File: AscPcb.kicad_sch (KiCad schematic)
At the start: 92 parts, among them J1 12402012E212A, J10 Conn_01x02_Pin, J11 Conn_01x02_Pin, J12 Conn_01x02_Pin, J13 Conn_01x02_Pin, J14 Conn_01x02_Pin, J15 Conn_01x02_Pin, J16 Conn_01x02_Pin, J17 Conn_01x02_Pin, J2 B2B-PH-K-S(LF)(SN), J3 Screw_Terminal_01x02, J4 Screw_Terminal_01x02, J5 Conn_01x15_Pin, J6 Conn_01x06_Pin, J7 Conn_01x02_Pin, J8 Conn_01x02_Pin, Q1 Q_NMOS_DGS, Q2 BC817, Q3 BC817, SW1 TL3305AF260QG, SW2 TL3305AF260QG, U1 BQ24040DSQR, U2 TLV75801PDRVR, U3 AP62300TWU, U4 LTC3625EDE_PBF, U5 ESP32-C3-WROOM-02-N4, U6 CP2102N-A02-GQFN24R, U7 BMI270, U8 74LVC1G07

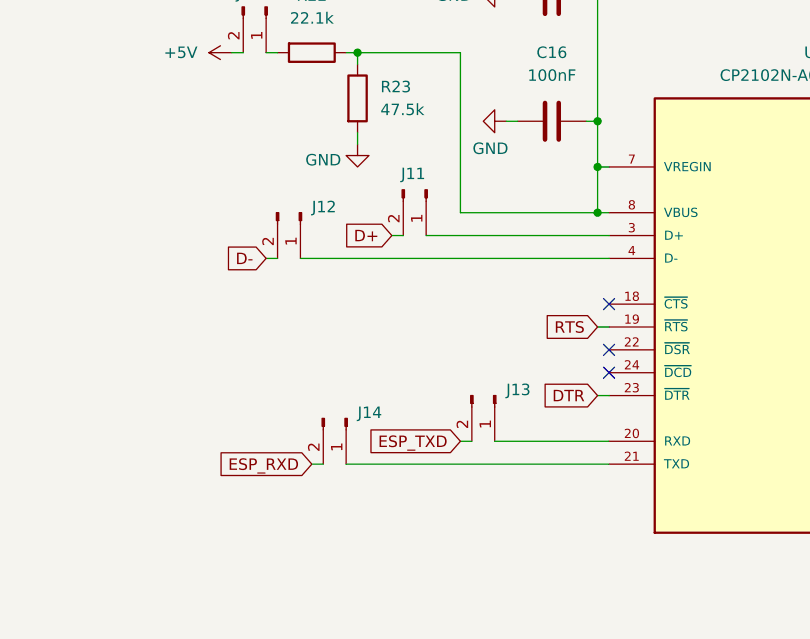
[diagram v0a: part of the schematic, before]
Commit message: first attempt at putting down traces
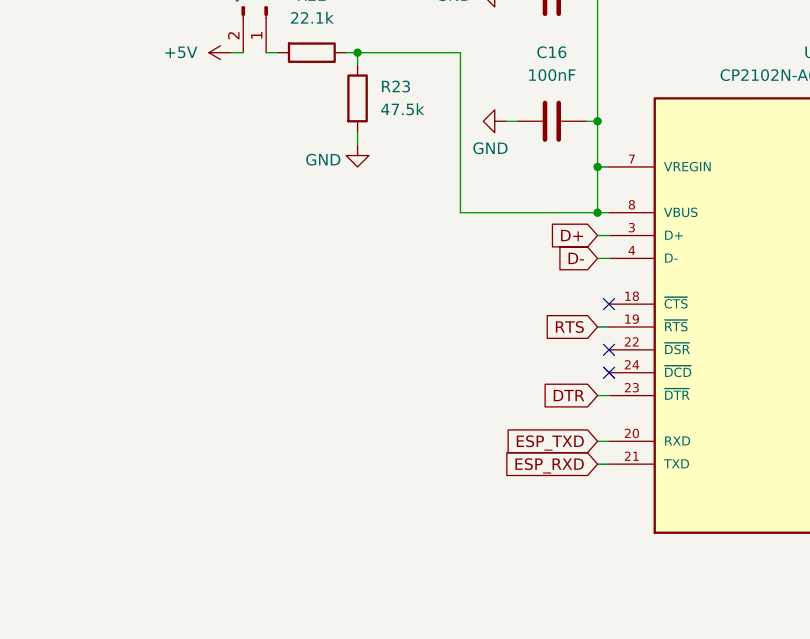
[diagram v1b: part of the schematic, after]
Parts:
- removed J11, J12, J13, J14: Conn_01x02_Pin, Connector_PinHeader_2.54mm:PinHeader_1x02_P2.54mm_Vertical, symbol Connector:Conn_01x02_Pin
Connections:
- net D+: now also U6.3 (D+)
- net D-: now also U6.4 (D-)
- net ESP_RXD: now also U6.21 (TXD)
- net ESP_TXD: now also U6.20 (RXD)

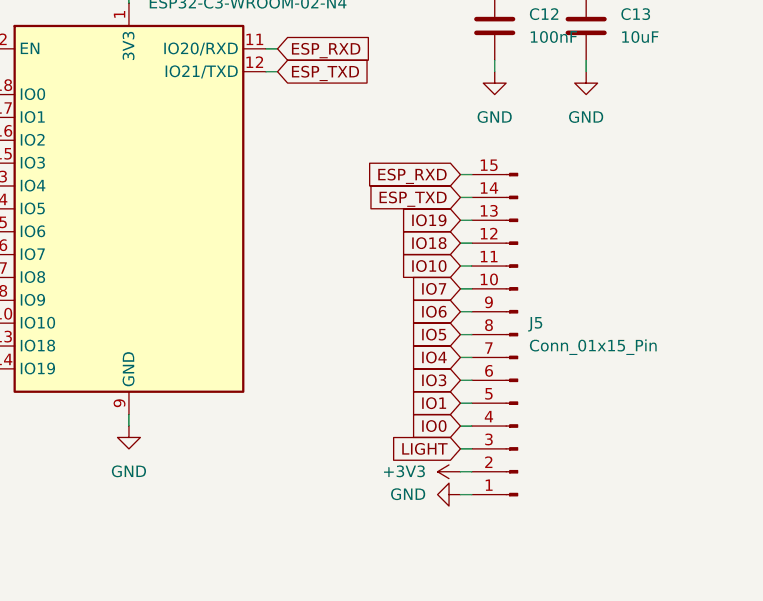
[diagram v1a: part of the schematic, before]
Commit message: routing done not gnd
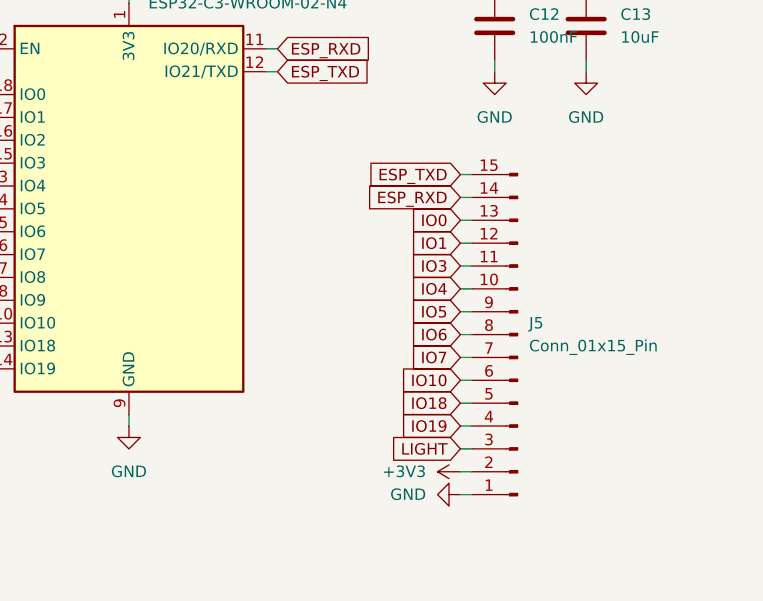
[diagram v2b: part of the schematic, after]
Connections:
- net ESP_RXD: now also J5.14 (Pin_14); no longer J5.15 (Pin_15)
- net ESP_TXD: now also J5.15 (Pin_15); no longer J5.14 (Pin_14)
- net IO0: now also J5.13 (Pin_13); no longer J5.4 (Pin_4)
- net IO1: now also J5.12 (Pin_12); no longer J5.5 (Pin_5)
- net IO10: now also J5.6 (Pin_6); no longer J5.11 (Pin_11)
- net IO18: now also J5.5 (Pin_5); no longer J5.12 (Pin_12)
- net IO19: now also J5.4 (Pin_4); no longer J5.13 (Pin_13)
- net IO3: now also J5.11 (Pin_11); no longer J5.6 (Pin_6)
- net IO4: now also J5.10 (Pin_10); no longer J5.7 (Pin_7)
- net IO5: now also J5.9 (Pin_9); no longer J5.8 (Pin_8)
- net IO6: now also J5.8 (Pin_8); no longer J5.9 (Pin_9)
- net IO7: now also J5.7 (Pin_7); no longer J5.10 (Pin_10)
